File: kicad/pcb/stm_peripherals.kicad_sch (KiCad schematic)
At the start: 3 parts, among them J4 SD Card, J6 Conn_01x40, U4 QSPI Flash

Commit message: Hub wired(?) + STM and ESP may boot already
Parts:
- J6: footprint (none) -> Connector_FFC-FPC:TE_4-1734839-0_1x40-1MP_P0.5mm_Horizontal
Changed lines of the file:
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@@
       (effects (font (size 1.27 1.27)) (justify left))
     )
-    (property "Footprint" "" (at 257.81 92.71 0)
+    (property "Footprint" "Connector_FFC-FPC:TE_4-1734839-0_1x40-1MP_P0.5mm_Horizontal" (at 257.81 92.71 0)
       (effects (font (size 1.27 1.27)) hide)
     )

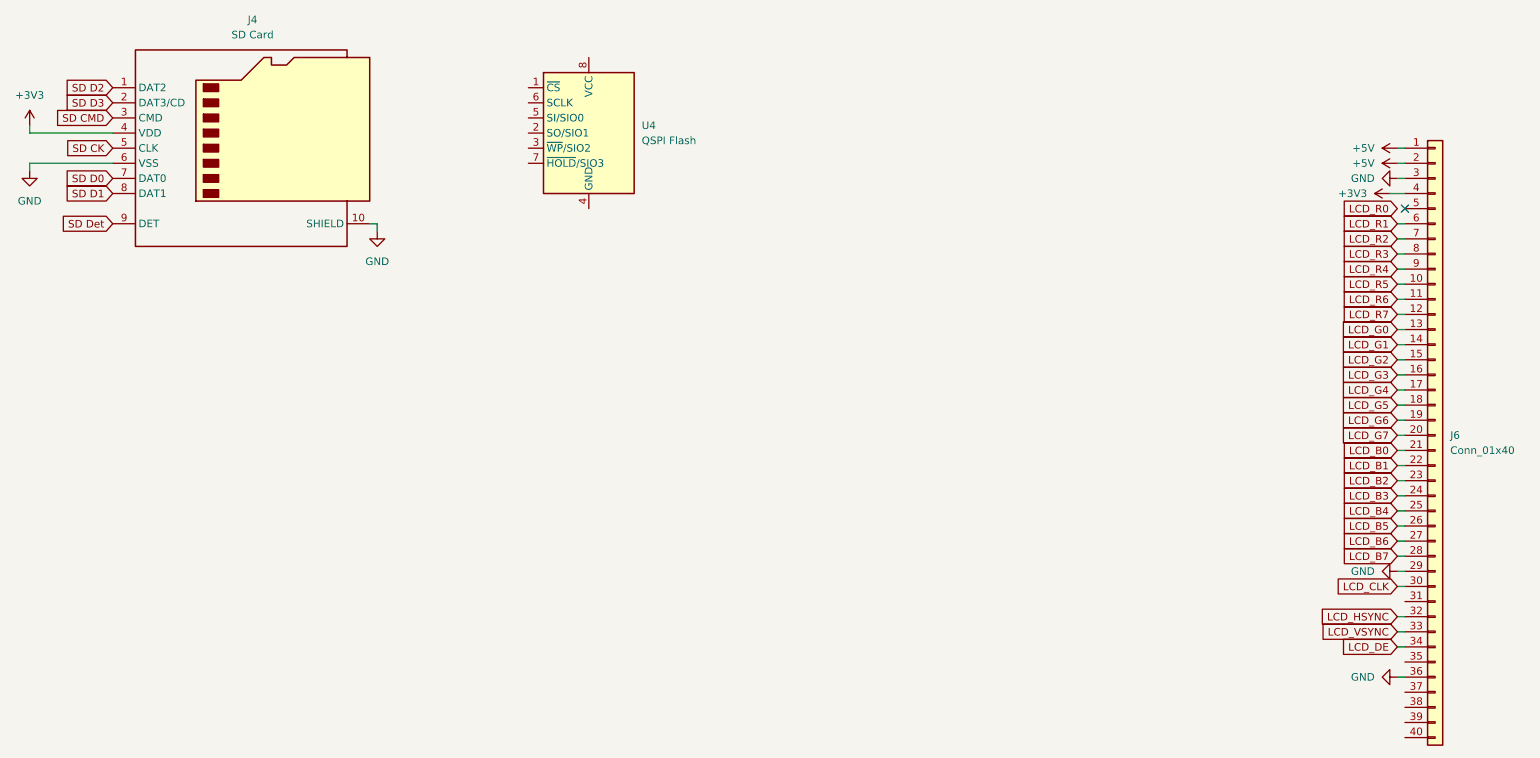
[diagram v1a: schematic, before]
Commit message: (WIP) Tracing v2
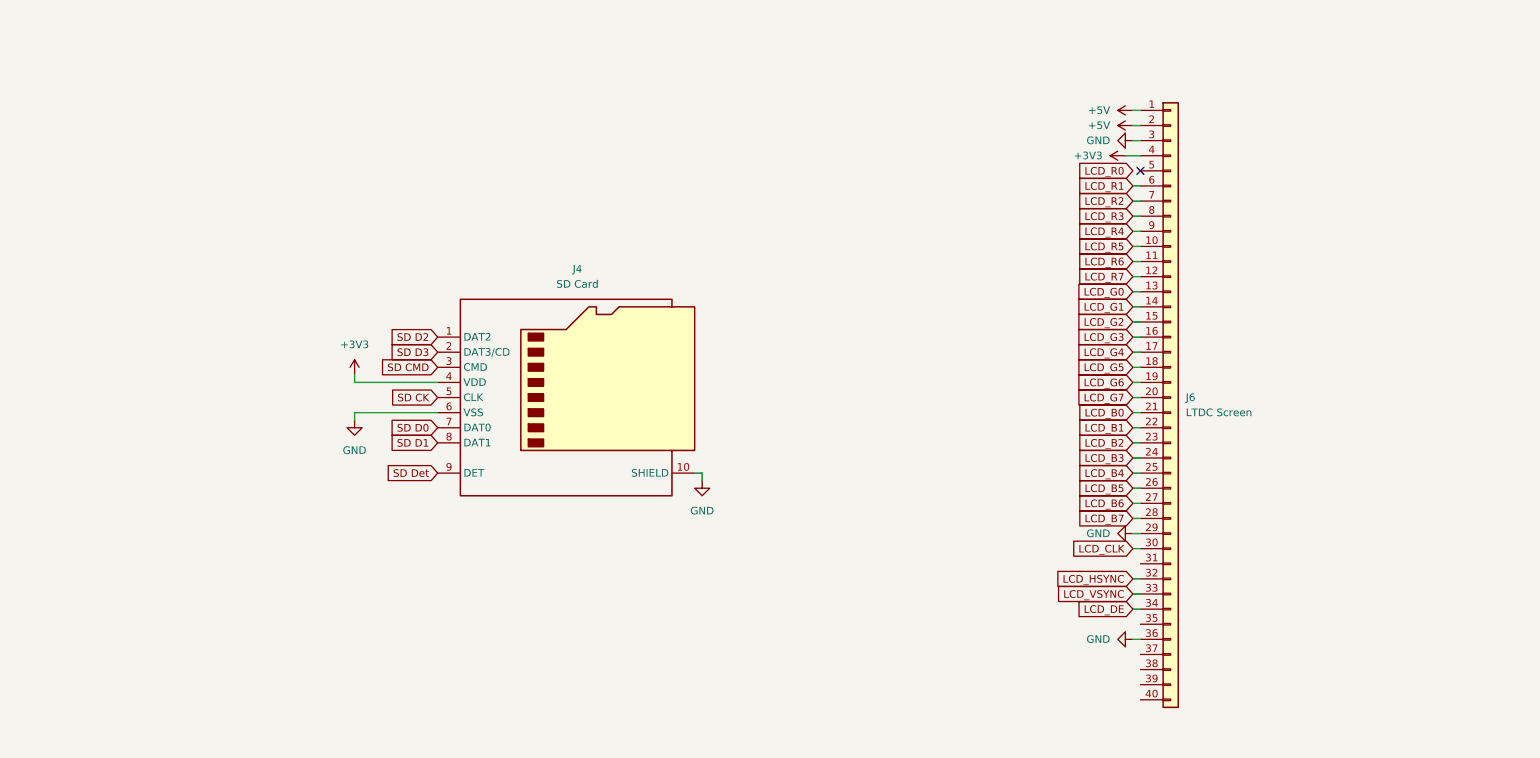
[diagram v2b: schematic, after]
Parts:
- removed U4: QSPI Flash, Package_SO:SOP-8_3.9x4.9mm_P1.27mm, symbol Memory_Flash:MX25R3235FM1xx1
- J4: footprint (none) -> Connector_Card:microSD_HC_Hirose_DM3AT-SF-PEJM5
- J6: value Conn_01x40 -> LTDC Screen
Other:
- moved on the sheet: J4, J6
